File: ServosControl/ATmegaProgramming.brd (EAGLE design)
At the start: 50 x 50 mm, 5 parts, among them U1 ATMEGA88PA-MU

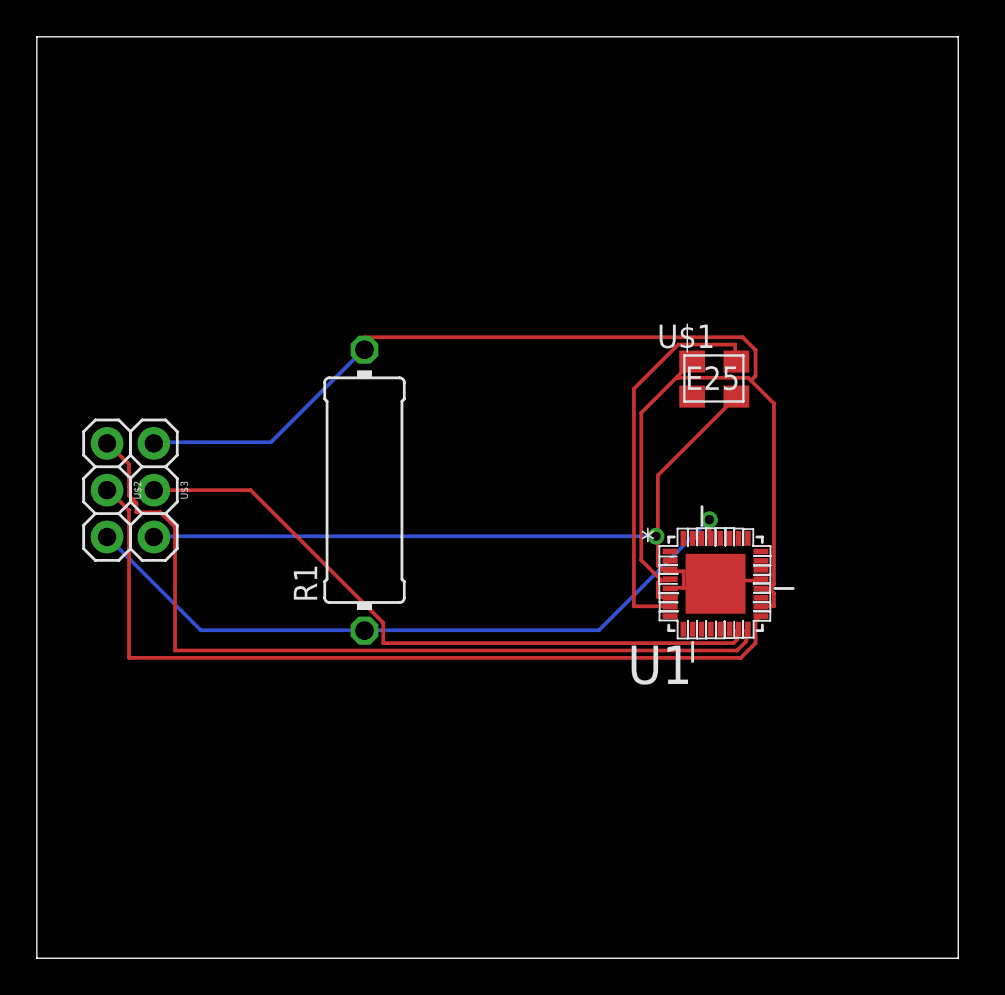
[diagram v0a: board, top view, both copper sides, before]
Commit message: Updating board
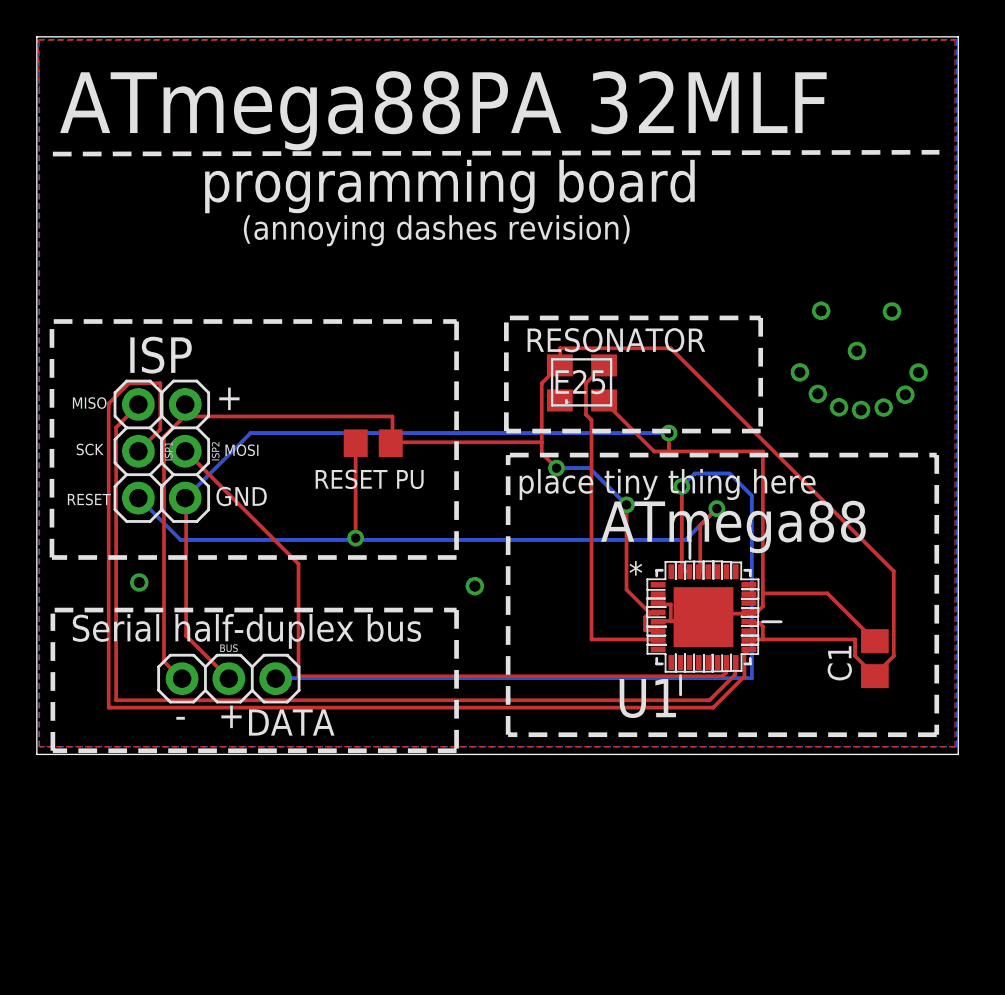
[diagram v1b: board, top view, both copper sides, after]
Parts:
- removed U$1: SG-310, RobotCampus:SG-310
- removed U$2, U$3: CONNEC_1X03, RobotCampus:CONNEC_1X03
- added BUS, ISP1, ISP2: CONNEC_1X03, RobotCampus:CONNEC_1X03
- added C1: 100nF, rhoban:C0805
- added RESONATOR: SG-310, RobotCampus:SG-310
- R1: device resistor:0414/15 -> rhoban:R0805
- U1: value ATMEGA88PA-MU -> (none)
- moved R1 2.59 mm to (18.3, 27.9), turned to 0 degrees
- moved U1 1.92 mm to (36.2, 18.5)
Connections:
- net CLOCK: now also RESONATOR.3; no longer U$1.3
- net DATA: now also BUS.3
- net GND: now also BUS.2, C1.2, ISP2.3, RESONATOR.2; no longer U$1.2, U$3.3
- net MISO: now also ISP1.1; no longer U$2.1
- net MOSI: now also ISP2.2; no longer U$3.2
- net RESET: now also ISP1.3; no longer U$2.3
- net SCK: now also ISP1.2; no longer U$2.2
- net VCC: now also BUS.1, C1.1, ISP2.1, RESONATOR.4; no longer U$1.4, U$3.1
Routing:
- net DATA: track 0.49 -> 45.5 mm, vias 0 -> 1
- net GND: track 46.1 -> 72.7 mm, vias 1 -> 13
- net VCC: track 71.4 -> 96.9 mm, vias 0 -> 2
- net SCK: track 45.6 -> 60.7 mm
- net MISO: track 45.5 -> 51.4 mm
- net RESET: track 38.4 -> 42.1 mm, vias 1 -> 2
- net MOSI: track 36.4 -> 38.6 mm
- net CLOCK: track 21.2 -> 19.0 mm
- added copper zone on layer 1, net GND
- added copper zone on layer 16, net GND
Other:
- board size 50 x 50 mm -> 50 x 38.9 mm
- board text added: "(annoying dashes revision)"
- board text added: "+"
- board text added: "-"
- board text added: "ATmega88"
- board text added: "ATmega88PA 32MLF"
- board text added: "DATA"
- board text added: "GND"
- board text added: "ISP"
- board text added: "MISO"
- board text added: "MOSI"
- board text added: "RESET"
- board text added: "RESET PU"
- board text added: "SCK"
- board text added: "Serial half-duplex bus"
- board text added: "place tiny thing here"
- board text added: "programming board"
